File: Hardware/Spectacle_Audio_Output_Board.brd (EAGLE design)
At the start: 25.4 x 55.9 mm, 86 parts, among them J4 AUDIO-JACK3, J5 AUDIO-JACK3, U1 CY8C4146LQI-S422, U2 3.3V, U3 3.3V, U4 AT25SF041-SOIC8, U5 VS1000, U6 SN74LVC1G66, U7 SN74LVC1G66, Y1 12MHz

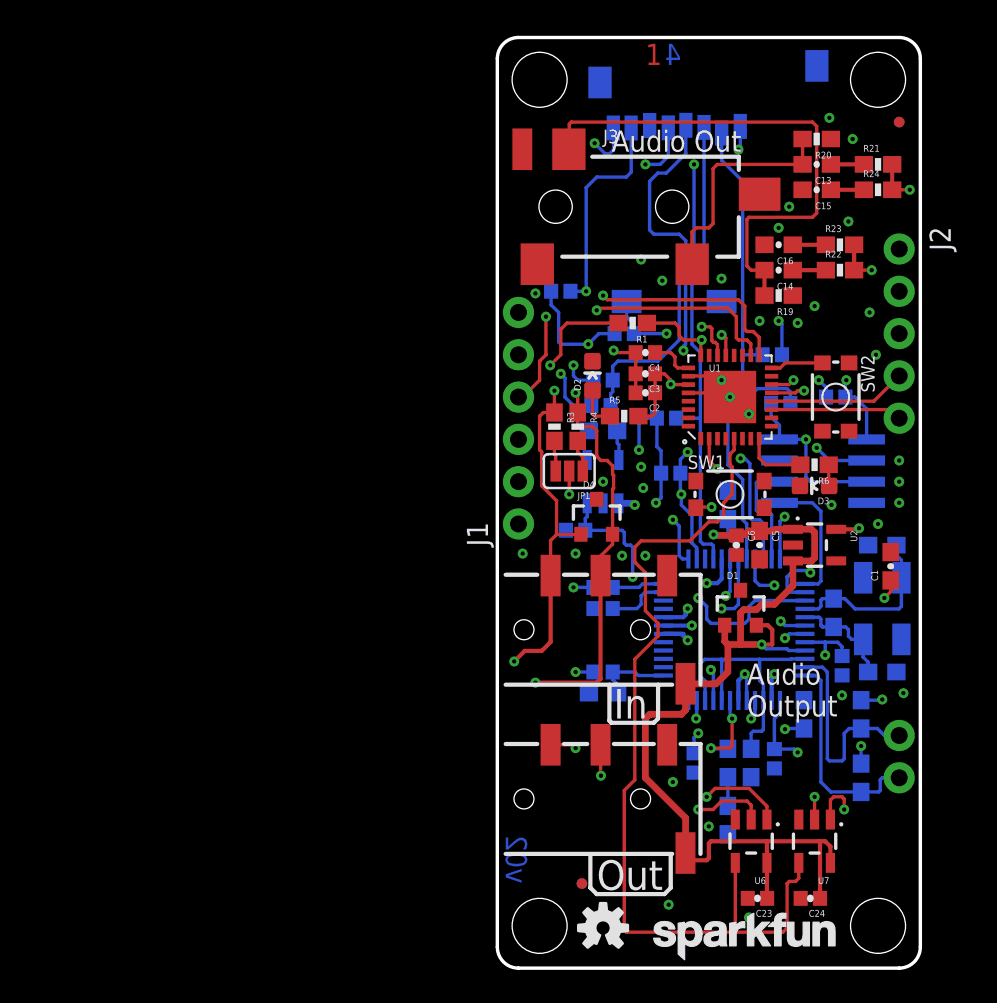
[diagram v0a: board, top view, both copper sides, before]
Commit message: Fixes from review
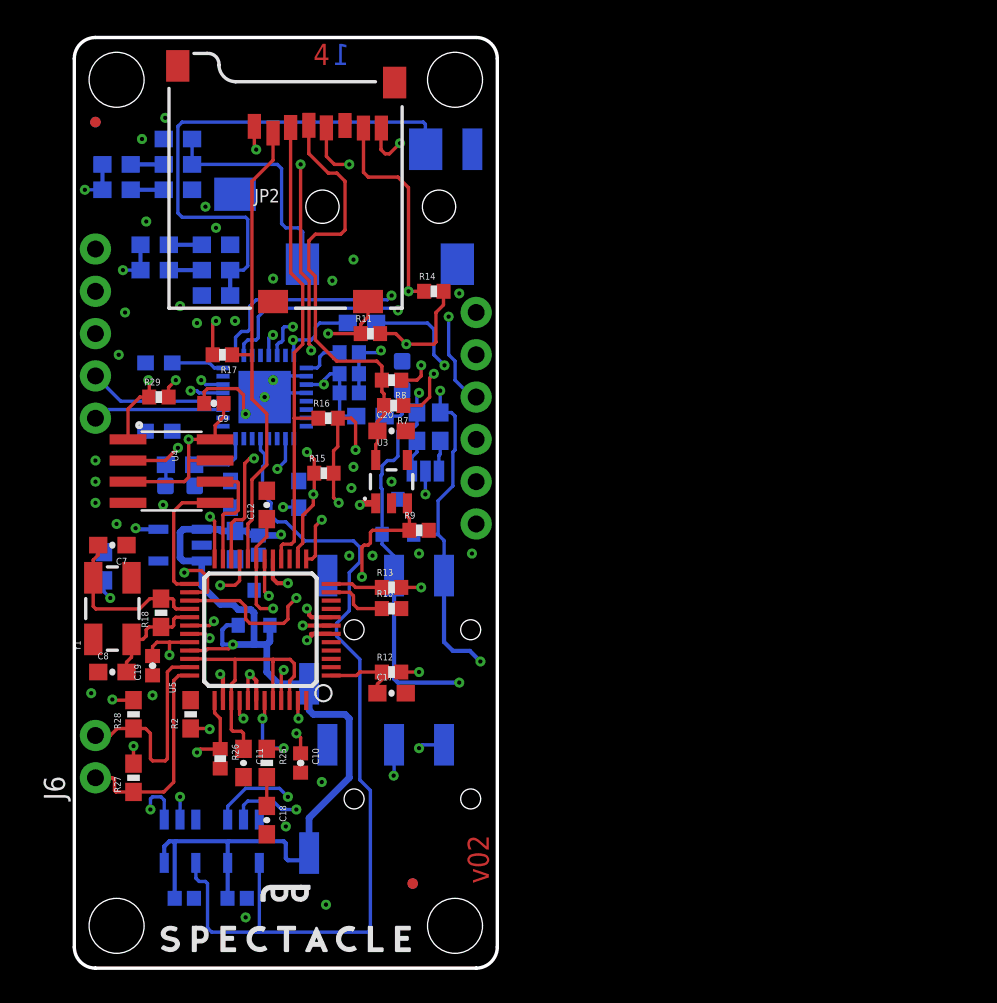
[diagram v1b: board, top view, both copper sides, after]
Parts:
- moved FRAME1 119.4 mm to (-59.7, 36.8), flipped to the bottom
- moved U$1 78.7 mm to (-39.4, 45.7), flipped to the bottom
- moved FD6 48.3 mm to (-24.1, 50.8), flipped to the top
- moved FD7 48.3 mm to (-24.1, 50.8), flipped to the bottom
- moved J2 48.3 mm to (-24.1, 43.2), flipped to the bottom
- moved J6 48.3 mm to (-24.1, 11.4), flipped to the top
- moved C1 47.2 mm to (-23.6, 24.1), flipped to the bottom
- moved C7 46.2 mm to (-23.1, 25.4), flipped to the top
- moved C8 46.2 mm to (-23.1, 17.8), flipped to the top
- moved Y1 46.2 mm to (-23.1, 21.6), flipped to the top
- moved H1 45.7 mm to (-22.9, 53.3), flipped to the bottom
- moved H3 45.7 mm to (-22.9, 2.54), flipped to the bottom
- moved R21 45.7 mm to (-22.9, 48.3), flipped to the bottom
- moved R24 45.7 mm to (-22.9, 46.7), flipped to the bottom
- moved R27 43.7 mm to (-21.8, 11.4), flipped to the top
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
